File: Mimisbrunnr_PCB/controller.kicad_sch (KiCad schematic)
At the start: 26 parts, among them J1 Conn_01x04_Female, J10 Conn_01x04_Female, SW1 SW_Push, SW2 SW_Push, SW3 SW_Push, U1 ESP32-WROOM-32, U3 MAX31856, U4 MAX31856, U5 MAX31856, U6 MAX31856, U7 MAX31856

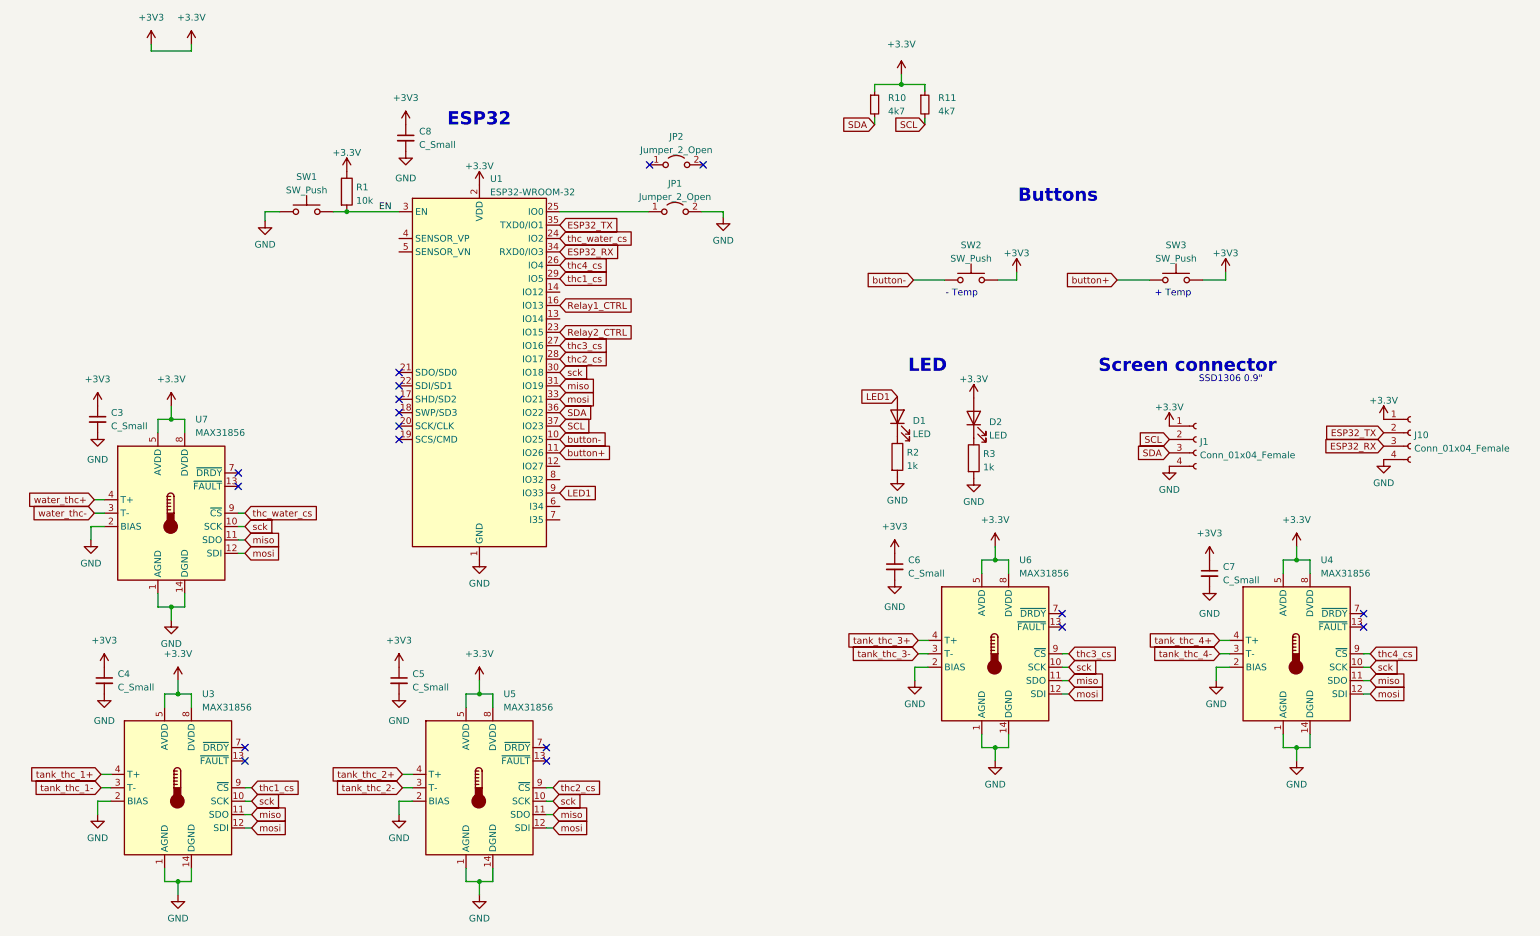
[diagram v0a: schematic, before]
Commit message: Improve style
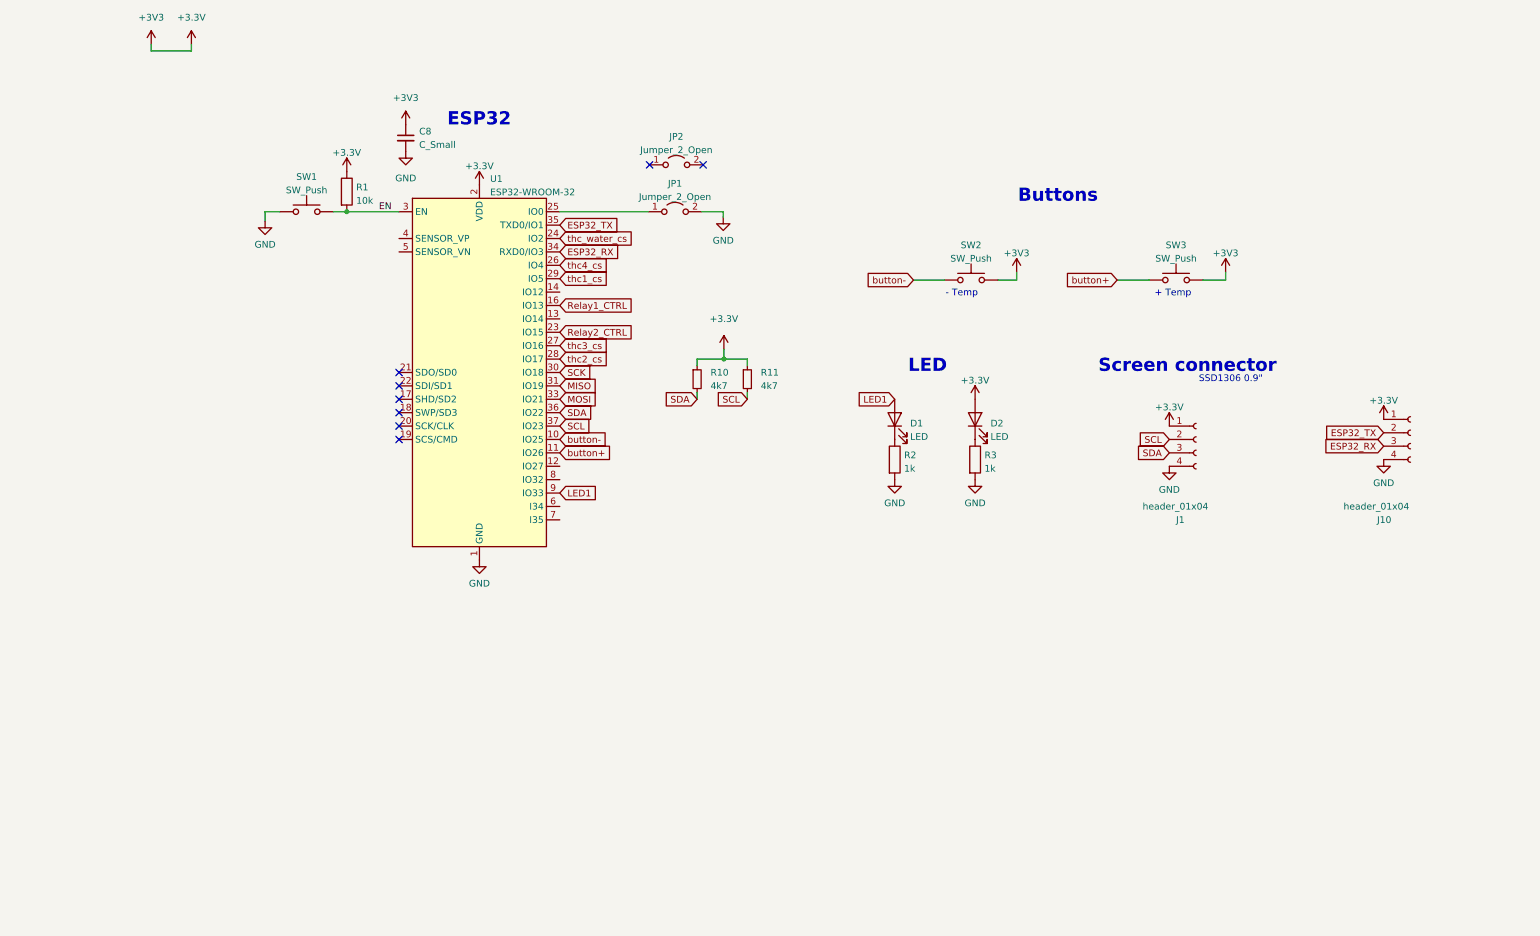
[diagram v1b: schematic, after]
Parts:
- removed C3, C4, C5, C6, C7: C_Small, Capacitor_SMD:C_0805_2012Metric, symbol Device:C_Small
- removed U3, U4, U5, U6, U7: MAX31856, Package_SO:TSSOP-14_4.4x5mm_P0.65mm, symbol Sensor_Temperature:MAX31856
- J1, J10: value Conn_01x04_Female -> header_01x04
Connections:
- net miso renamed MISO
- net mosi renamed MOSI
- net sck renamed SCK
- no-connect marks 18 -> 8
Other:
- moved on the sheet: D1, R10, R11, R2
